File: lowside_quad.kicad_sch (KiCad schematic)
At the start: 4 parts, among them U201 VNLD5160, U202 VNLD5160

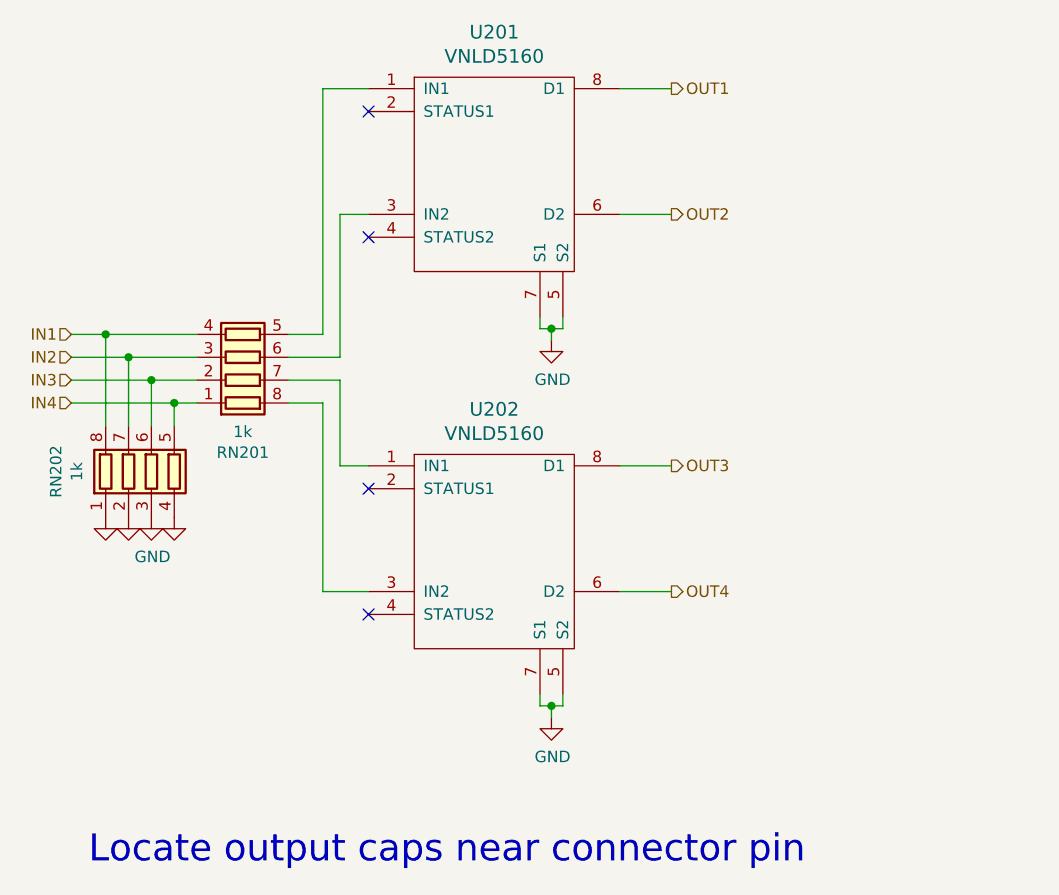
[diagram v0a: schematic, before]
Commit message: Packaged LS13-16 with the flyback diodes
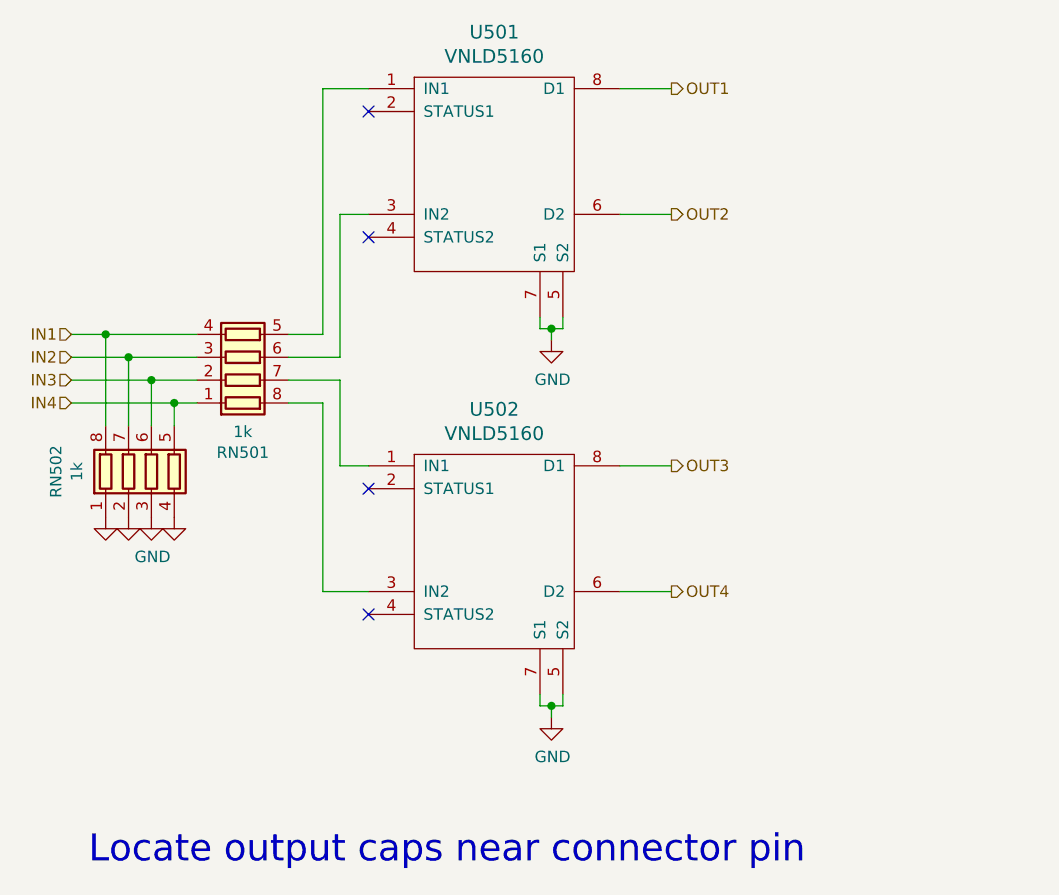
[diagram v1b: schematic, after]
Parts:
- renumbered RN201 to RN501, RN202 to RN502, U201 to U501, U202 to U502
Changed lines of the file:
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@@
   (symbol (lib_id "vnld5090:VNLD5090") (at 106.045 51.435 0)
     (in_bom yes) (on_board yes)
-    (property "Reference" "U201" (id 0) (at 106.045 35.0012 0)
+    (property "Reference" "U501" (id 0) (at 106.045 35.0012 0)
       (effects (font (size 1.524 1.524)))
     )
@@
   (symbol (lib_id "vnld5090:VNLD5090") (at 106.045 93.345 0)
     (in_bom yes) (on_board yes)
-    (property "Reference" "U202" (id 0) (at 106.045 76.9112 0)
+    (property "Reference" "U502" (id 0) (at 106.045 76.9112 0)
       (effects (font (size 1.524 1.524)))
     )
@@
   (symbol (lib_id "Device:R_Pack04") (at 78.105 71.12 270) (mirror x)
     (in_bom yes) (on_board yes)
-    (property "Reference" "RN201" (id 0) (at 78.105 81.7118 90))
+    (property "Reference" "RN501" (id 0) (at 78.105 81.7118 90))
     (property "Value" "1k" (id 1) (at 78.105 79.4004 90))
     (property "Footprint" "Resistor_SMD:R_Array_Convex_4x0603" (id 2) (at 78.105 64.135 90)
@@
   (symbol (lib_id "Device:R_Pack04") (at 67.945 83.82 0)
     (in_bom yes) (on_board yes)
-    (property "Reference" "RN202" (id 0) (at 57.3532 83.82 90))
+    (property "Reference" "RN502" (id 0) (at 57.3532 83.82 90))
     (property "Value" "1k" (id 1) (at 59.6646 83.82 90))
     (property "Footprint" "Resistor_SMD:R_Array_Convex_4x0603" (id 2) (at 74.93 83.82 90)

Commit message: Nearly finished routing
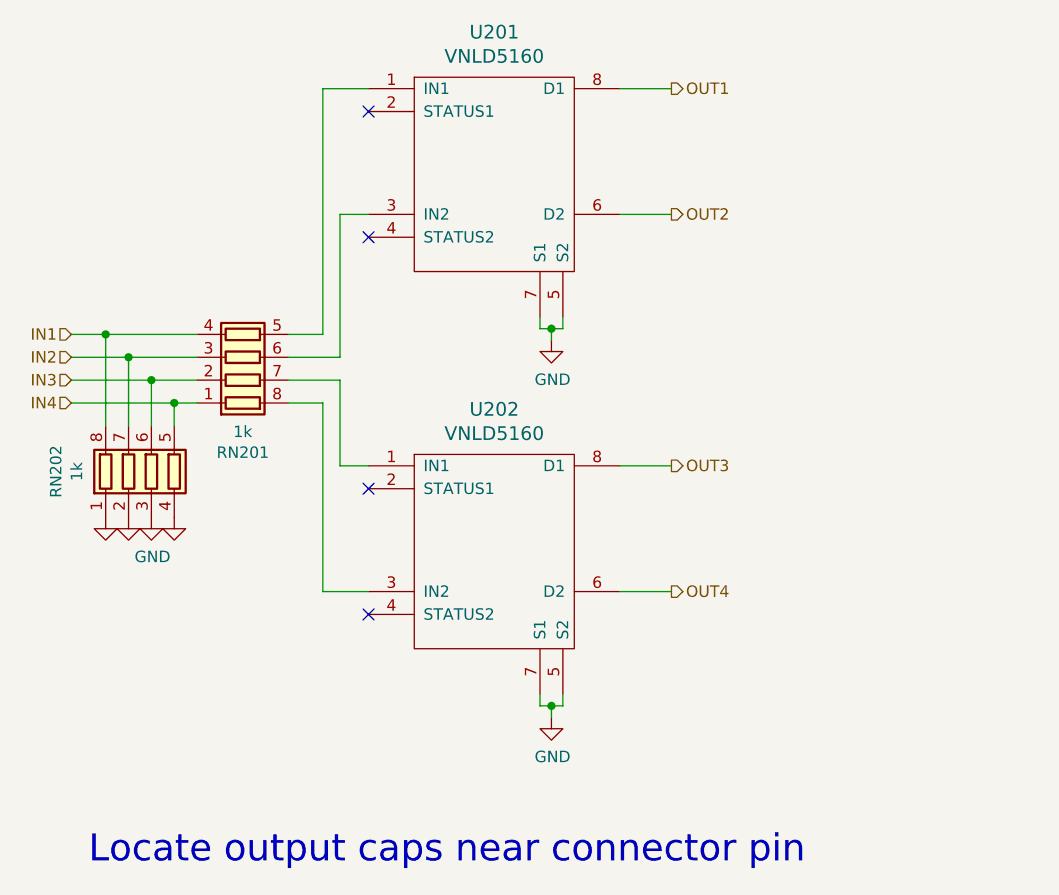
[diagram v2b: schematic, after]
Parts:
- renumbered RN501 to RN201, RN502 to RN202, U501 to U201, U502 to U202
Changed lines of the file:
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@@
   (symbol (lib_id "vnld5090:VNLD5090") (at 106.045 51.435 0)
     (in_bom yes) (on_board yes)
-    (property "Reference" "U501" (id 0) (at 106.045 35.0012 0)
+    (property "Reference" "U201" (id 0) (at 106.045 35.0012 0)
       (effects (font (size 1.524 1.524)))
     )
@@
   (symbol (lib_id "vnld5090:VNLD5090") (at 106.045 93.345 0)
     (in_bom yes) (on_board yes)
-    (property "Reference" "U502" (id 0) (at 106.045 76.9112 0)
+    (property "Reference" "U202" (id 0) (at 106.045 76.9112 0)
       (effects (font (size 1.524 1.524)))
     )
@@
   (symbol (lib_id "Device:R_Pack04") (at 78.105 71.12 270) (mirror x)
     (in_bom yes) (on_board yes)
-    (property "Reference" "RN501" (id 0) (at 78.105 81.7118 90))
+    (property "Reference" "RN201" (id 0) (at 78.105 81.7118 90))
     (property "Value" "1k" (id 1) (at 78.105 79.4004 90))
     (property "Footprint" "Resistor_SMD:R_Array_Convex_4x0603" (id 2) (at 78.105 64.135 90)
@@
   (symbol (lib_id "Device:R_Pack04") (at 67.945 83.82 0)
     (in_bom yes) (on_board yes)
-    (property "Reference" "RN502" (id 0) (at 57.3532 83.82 90))
+    (property "Reference" "RN202" (id 0) (at 57.3532 83.82 90))
     (property "Value" "1k" (id 1) (at 59.6646 83.82 90))
     (property "Footprint" "Resistor_SMD:R_Array_Convex_4x0603" (id 2) (at 74.93 83.82 90)
